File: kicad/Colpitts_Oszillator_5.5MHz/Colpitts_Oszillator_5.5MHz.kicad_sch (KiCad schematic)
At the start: 15 parts, among them Q1 2N3904

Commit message: Remove KiCad .history repo from tracking
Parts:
- C1: footprint 47pF -> (none)
- R3: footprint 51Ohm -> (none)
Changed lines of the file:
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@@
 			)
 		)
-		(property "Footprint" "51Ohm"
+		(property "Footprint" ""
 			(at 129.032 120.65 90)
 			(hide yes)
@@
 			)
 		)
-		(property "Footprint" "47pF"
+		(property "Footprint" ""
 			(at 180.0352 82.55 0)
 			(hide yes)

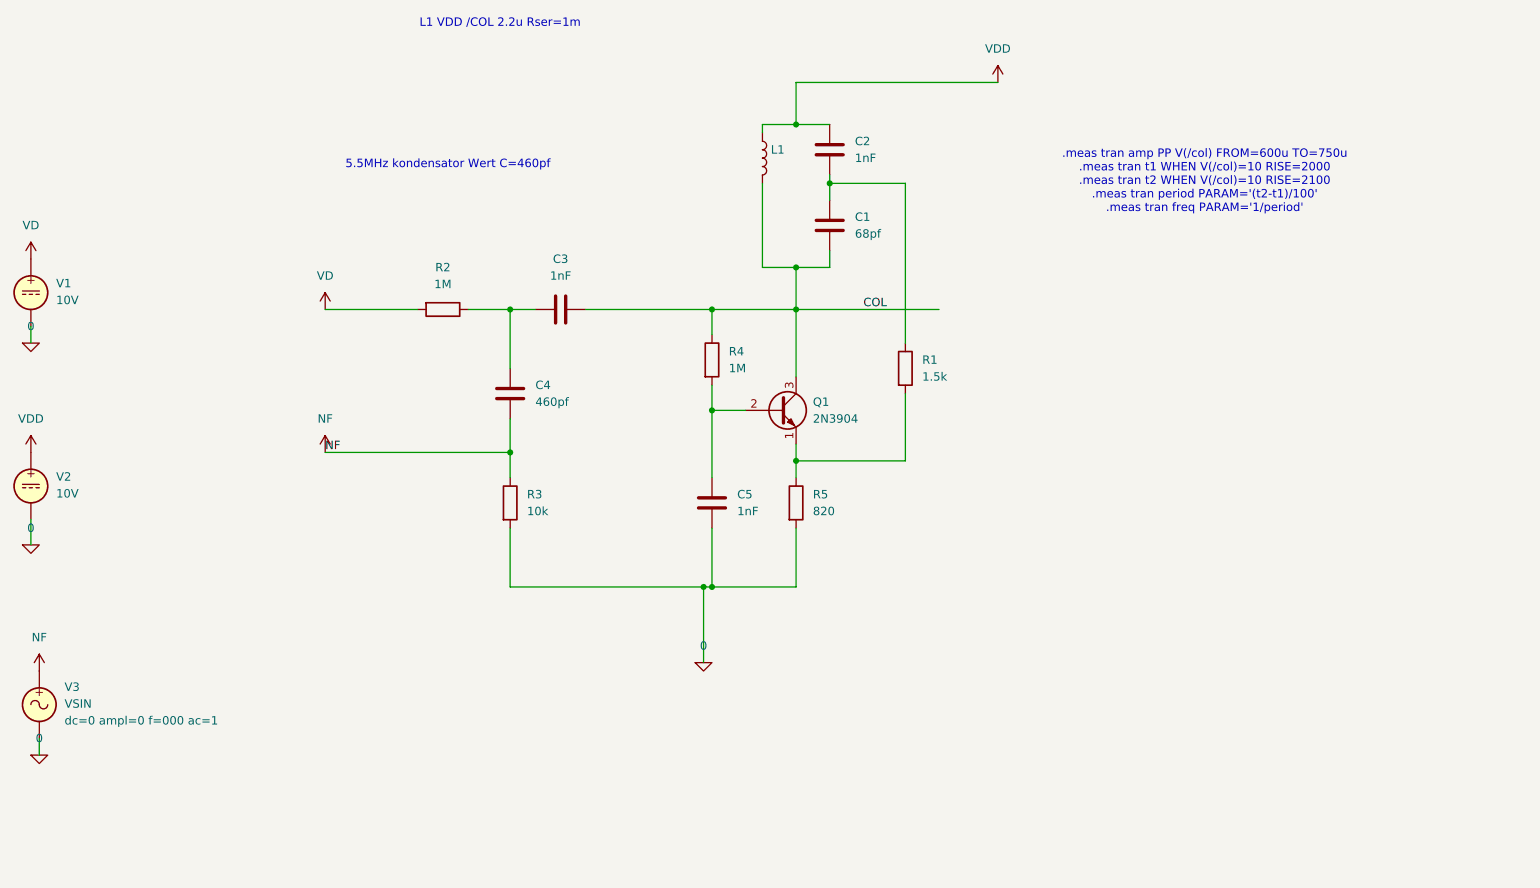
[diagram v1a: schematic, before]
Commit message: Aktueller Stand
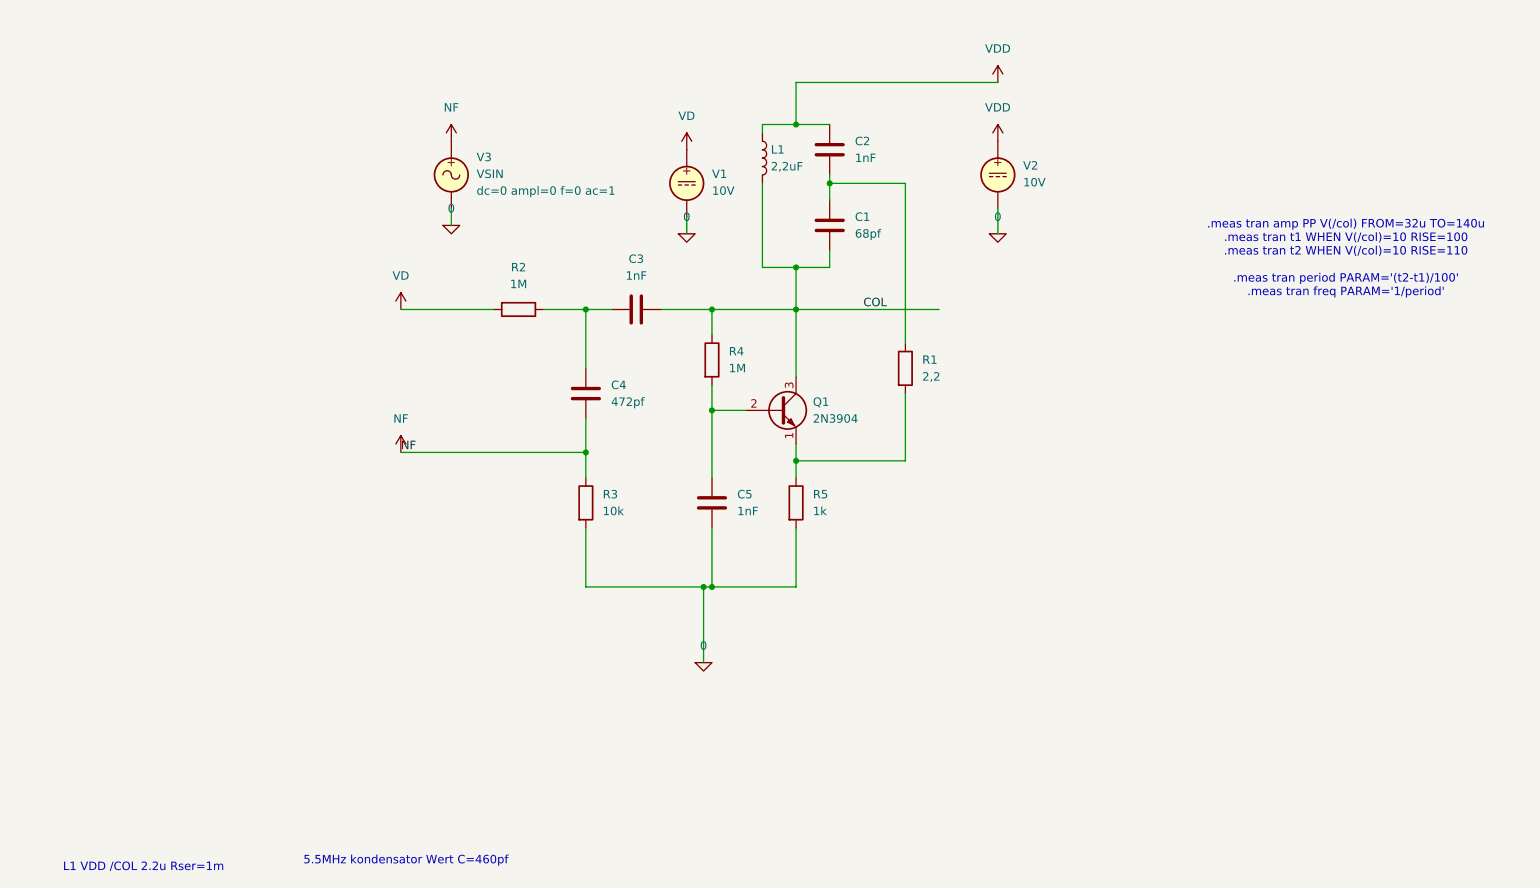
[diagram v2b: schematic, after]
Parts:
- C1: footprint (none) -> 47pF
- C4: value 460pf -> 472pf
- L1: value (none) -> 2,2uF
- R1: value 1.5k -> 2,2
- R3: footprint (none) -> 51Ohm
- R5: value 820 -> 1k
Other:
- note added: ".meas tran amp PP V(/col) FROM=32u TO=140u .meas tran t1 WHEN V(/col)=10 RISE=100 .meas tran t2 WHEN V(/col)=10 RISE=110 .meas tran period PARAM='(t2-t1)/100' .meas tran freq PARAM='1/period'"
- note removed: ".meas tran amp PP V(/col) FROM=600u TO=750u .meas tran t1 WHEN V(/col)=10 RISE=2000 .meas tran t2 WHEN V(/col)=10 RISE=2100 .meas tran period PARAM='(t2-t1)/100' .meas tran freq PARAM='1/period'"
- moved on the sheet: C3, C4, R2, R3, V1, V2, V3
